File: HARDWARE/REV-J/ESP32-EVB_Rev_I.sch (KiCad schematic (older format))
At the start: 154 parts, among them CON1 TB3 DG306-5.0-3P, CON2 TB3 DG306-5.0-3P, Q1 BC817-40(SOT23), Q2 BC817-40(SOT23), Q3 Q12MHz/20pF/30ppm/2P/HC-49SM(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, Q4 BC817-40(SOT23), Q5 BC817-40(SOT23), Q6 BC817, Q7 BC817-40(SOT23), U1 BL4054B-42TPRN(SOT23-5), U10 BAT54C(SOT23-3), U2 SY8089AAAC(SOT23-5), U3 ESP-WROOM-32, U4 LAN8710A-EZC(QFN32), U5 CH340T(SSOP20W), U6 MCP2562-E/SN(SOIC-8_150mil), U7 RPM7236-H8, U8 NCP303LSN27T1G(SOT-23-5), U9 BAT54C(SOT23-3)

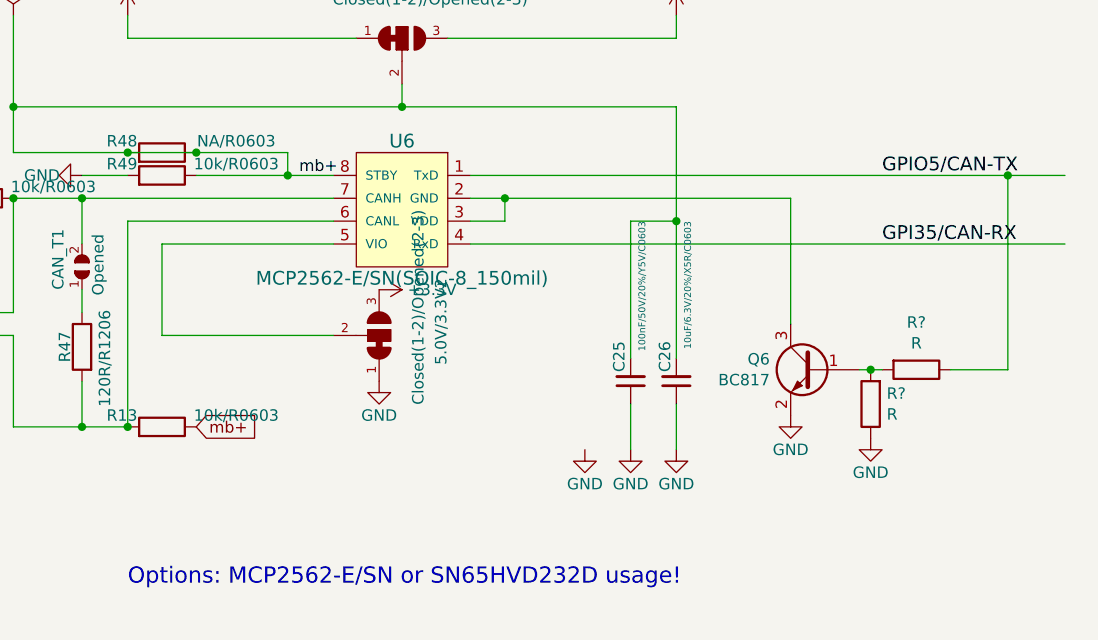
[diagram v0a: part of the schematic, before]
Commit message: Update ESP32-EVB_Rev_I-cache.lib, ESP32-EVB_Rev_I.kicad_pcb, and 4 more files...
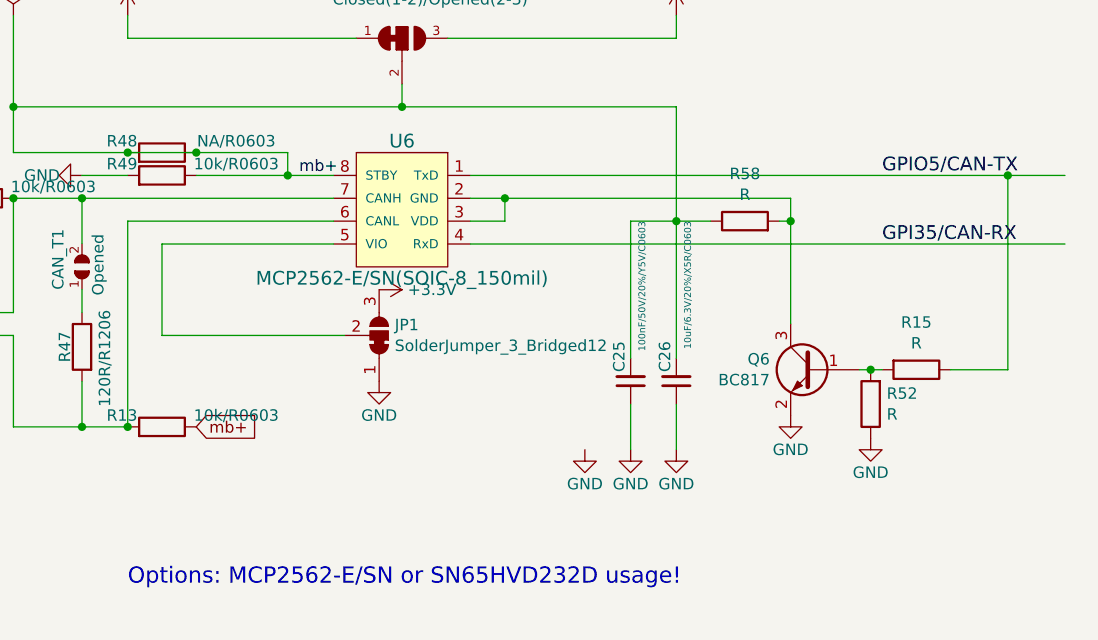
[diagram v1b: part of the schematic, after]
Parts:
- removed 5.0V/3.3V2: Closed(1-2)/Opened(2-3), OLIMEX_Jumpers-FP:SJ_2_SMALL_12_TIED, symbol ESP32-EVB_Rev_I:SJ2W_Closed(1-2)
- added JP1: SolderJumper_3_Bridged12, Jumper:SolderJumper-3_P1.3mm_Bridged2Bar12_Pad1.0x1.5mm_NumberLabels, symbol Jumper:SolderJumper_3_Bridged12
- added R58: R, Resistor_SMD:R_0603_1608Metric, symbol Device:R
- gave numbers to parts that had none: 2
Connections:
- wire segments 697 -> 700
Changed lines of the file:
@@
-$EndComp
-$Comp
-L ESP32-EVB_Rev_I:SJ2W_Closed(1-2) 5.0V/3.3V2
-U 1 1 61B60BDC
-P 12600 14400
-F 0 "5.0V/3.3V2" V 12900 14150 50  0000 L BNN
-F 1 "Closed(1-2)/Opened(2-3)" V 12800 13850 50  0000 L BNN
-F 2 "OLIMEX_Jumpers-FP:SJ_2_SMALL_12_TIED" H 12630 14550 20  0001 C CNN
-F 3 "" H 12600 14400 60  0000 C CNN
-	1    12600 14400
-	1    0    0    1
 $EndComp
 $Comp
@@
 	1    0    0    -1
 $EndComp
-Wire Wire Line
-	12400 14400 11650 14400
 Wire Wire Line
 	11650 14400 11650 14000
@@
 	13150 13800 14400 13800
 Wire Wire Line
-	14400 13800 14400 14350
+	14400 13800 14400 13900
 Connection ~ 13150 13800
 $Comp
@@
 	14700 14550 14750 14550
 $Comp
-L Device:R R?
+L Device:R R15
 U 1 1 614C248B
 P 14950 14550
-F 0 "R?" V 14743 14550 50  0000 C CNN
+F 0 "R15" V 14743 14550 50  0000 C CNN
 F 1 "R" V 14834 14550 50  0000 C CNN
 F 2 "Resistor_SMD:R_0603_1608Metric" V 14880 14550 50  0001 C CNN
@@
 $EndComp
 $Comp
-L Device:R R?
+L Device:R R52
 U 1 1 614C4787
 P 14750 14700
-F 0 "R?" H 14680 14654 50  0000 R CNN
+F 0 "R52" H 14680 14654 50  0000 R CNN
 F 1 "R" H 14680 14745 50  0000 R CNN
 F 2 "Resistor_SMD:R_0603_1608Metric" V 14680 14700 50  0001 C CNN
@@
 Wire Wire Line
 	14750 14550 14800 14550
+$Comp
+L Device:R R58
+U 1 1 614C9259
+P 14200 13900
+F 0 "R58" V 14407 13900 50  0000 C CNN
+F 1 "R" V 14316 13900 50  0000 C CNN
+F 2 "Resistor_SMD:R_0603_1608Metric" V 14130 13900 50  0001 C CNN
+F 3 "~" H 14200 13900 50  0001 C CNN
+	1    14200 13900
+	0    -1   -1   0
+$EndComp
+Wire Wire Line
+	14050 13900 13900 13900
+Wire Wire Line
+	14350 13900 14400 13900
+Connection ~ 14400 13900
+Wire Wire Line
+	14400 13900 14400 14350
+$Comp
+L Jumper:SolderJumper_3_Bridged12 JP1
+U 1 1 616705BA
+P 12600 14400
+F 0 "JP1" V 12646 14468 50  0000 L CNN
+F 1 "SolderJumper_3_Bridged12" V 12555 14468 50  0000 L CNN
+F 2 "Jumper:SolderJumper-3_P1.3mm_Bridged2Bar12_Pad1.0x1.5mm_NumberLabels" H 12600 14400 50  0001 C CNN
+F 3 "~" H 12600 14400 50  0001 C CNN
+	1    12600 14400
+	0    1    -1   0
+$EndComp
+Wire Wire Line
+	11650 14400 12450 14400
 $EndSCHEMATC
